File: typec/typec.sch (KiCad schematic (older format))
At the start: 26 parts, among them U1 TPD6E05U06-USON, U2 TPD4E05U06-USON, U3 TPS62081-WSON, U4 TPD4E05U06-USON, U5 TPS74801-VSON, U6 TUSB212-X2QFN

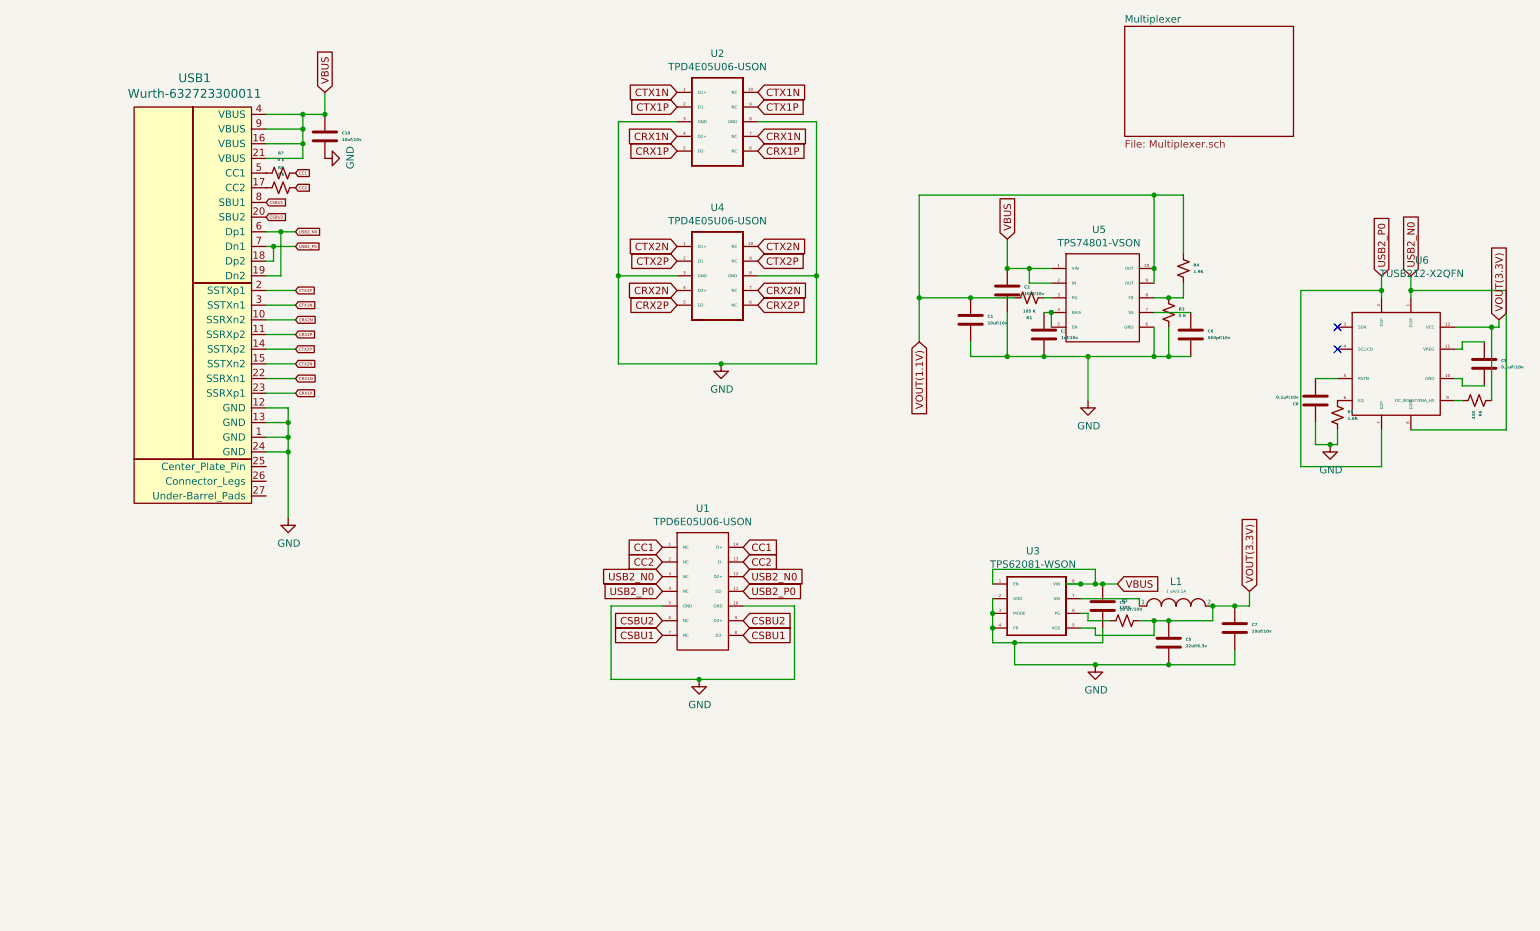
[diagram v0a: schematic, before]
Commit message: updated
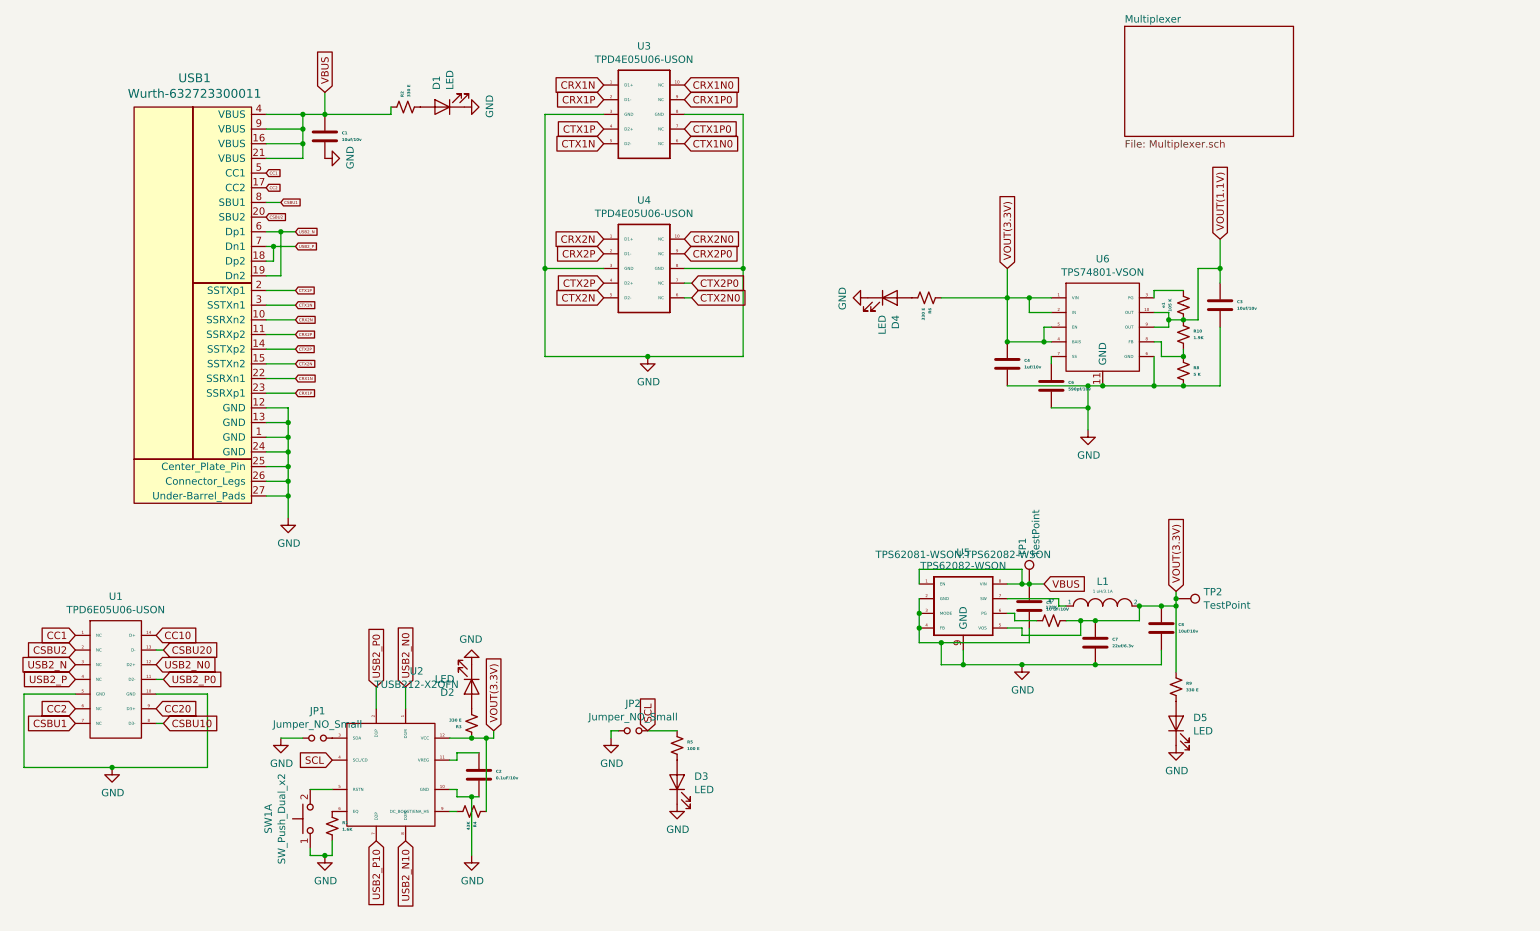
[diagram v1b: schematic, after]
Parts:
- removed C1: 10uf/10v, Capacitor_SMD:C_0805_2012Metric, symbol Device:C
- removed C9: 0.1uF/10v, Capacitor_SMD:C_0402_1005Metric, symbol Device:C
- removed U3: TPS62081-WSON, TPS62081-WSON:TPS62081-WSON, symbol typec-rescue:TPS62081-WSON-TPS62081-WSON
- removed U5: TPS74801-VSON, TPS74801-VSON:TPS74801-VSON, symbol typec-rescue:TPS74801-VSON-TPS74801-VSON
- removed U6: TUSB212-X2QFN, TUSB212-X2QFN:TUSB212-X2QFN, symbol TUSB212-X2QFN:TUSB212-X2QFN
- added D1, D2, D3, D4, D5: LED, LED_SMD:LED_0402_1005Metric, symbol Device:LED
- added JP1, JP2: Jumper_NO_Small, Connector_PinHeader_1.00mm:PinHeader_1x02_P1.00mm_Vertical, symbol Device:Jumper_NO_Small
- added R10: 1.9K, Resistor_SMD:R_0402_1005Metric, symbol Device:R_Small_US
- added R9: 330 E, Resistor_SMD:R_0402_1005Metric, symbol Device:R_Small_US
- added SW1: SW_Push_Dual_x2, Button_Switch_THT:SW_DIP_SPSTx01_Slide_6.7x4.1mm_W7.62mm_P2.54mm_LowProfile, symbol Switch:SW_Push_Dual_x2
- added TP1, TP2: TestPoint, TestPoint:TestPoint_THTPad_2.0x2.0mm_Drill1.0mm, symbol Connector:TestPoint
- added U2: TUSB212-X2QFN, TUSB212-X2QFN:TUSB212-X2QFN, symbol TUSB212-X2QFN:TUSB212-X2QFN
- added U5: TPS62082-WSON, TPS62081-WSON:TPS62082-WSON, symbol typec-rescue:TPS62082-WSON
- added U6: TPS74801-VSON, TPS74801-VSON:TPS74801-VSON, symbol TPS74801-VSON:TPS74801-VSON
- added e1: 105 K, Resistor_SMD:R_0201_0603Metric, symbol Device:R_Small_US
- C2: value 10uf/10v -> 0.1uF/10v; footprint Capacitor_SMD:C_0805_2012Metric -> Capacitor_SMD:C_0402_1005Metric
- C3: value 1uf/10v -> 10uf/10v
- C4: value 10 uF/10V -> 1uf/10v; footprint Capacitor_SMD:C_0805_2012Metric -> Capacitor_SMD:C_0603_1608Metric
- C5: value 22uf/6.3v -> 10 uF/10V; footprint Capacitor_SMD:C_0805_2012Metric -> Capacitor_SMD:C_0603_1608Metric
- C6: value 560pf/10v -> 590pf/10v; footprint Capacitor_SMD:C_0402_1005Metric -> Capacitor_SMD:C_0201_0603Metric
- C7: value 10uf/10v -> 22uf/6.3v; footprint Capacitor_SMD:C_0805_2012Metric -> Capacitor_SMD:C_0603_1608Metric
- C8: value 0.1uF/10v -> 10uf/10v; footprint Capacitor_SMD:C_0402_1005Metric -> Capacitor_SMD:C_0603_1608Metric
- R1: value 105 K -> 1.6K; footprint Resistor_SMD:R_0805_2012Metric -> Resistor_SMD:R_0201_0603Metric
- R2: value 178K -> 330 E; footprint Resistor_SMD:R_0805_2012Metric -> Resistor_SMD:R_0402_1005Metric
- R3: value 5 K -> 330 E; footprint Resistor_SMD:R_0805_2012Metric -> Resistor_SMD:R_0201_0603Metric
- R4: value 1.9K -> 43K; footprint Resistor_SMD:R_0805_2012Metric -> Resistor_SMD:R_0201_0603Metric
- R5: value 1.6K -> 100 E; footprint Resistor_SMD:R_0805_2012Metric -> Resistor_SMD:R_0402_1005Metric
- R6: value 43K -> 330 E; footprint Resistor_SMD:R_0805_2012Metric -> Resistor_SMD:R_0402_1005Metric
- R7: value 0 E -> 178K; footprint Resistor_SMD:R_0805_2012Metric -> Resistor_SMD:R_0402_1005Metric
- R8: value 0 E -> 5 K; footprint Resistor_SMD:R_0805_2012Metric -> Resistor_SMD:R_0402_1005Metric
- renumbered C10 to C1, U2 to U3
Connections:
- net CC1: now also USB1.5 (CC1); no longer R7.1, U1.14 (D+)
- net CC2: now also U1.6 (NC), USB1.17 (CC2); no longer R8.1, U1.13 (D-), U1.2 (NC)
- net CRX1N: now also U3.1 (D1+); no longer U3.4 (D2+), U3.7 (NC)
- net CRX1P: now also U3.2 (D1-); no longer U3.5 (D2-), U3.6 (NC)
- net CRX2N: now also U4.1 (D1+); no longer U4.4 (D2+), U4.7 (NC)
- net CRX2P: now also U4.2 (D1-); no longer U4.5 (D2-), U4.6 (NC)
- net CSBU1: no longer U1.8 (D3-)
- net CSBU2: now also U1.2 (NC); no longer U1.6 (NC), U1.9 (D3+)
- net CTX1N: now also U3.5 (D2-); no longer U3.1 (D1+), U3.10 (NC)
- net CTX1P: now also U3.4 (D2+); no longer U3.2 (D1-), U3.9 (NC)
- net CTX2N: now also U4.5 (D2-); no longer U4.1 (D1+), U4.10 (NC)
- net CTX2P: now also U4.4 (D2+); no longer U4.2 (D1-), U4.9 (NC)
- net GND: now also C8.2, R1.2, R8.1, USB1.25 (Center_Plate_Pin), USB1.26 (Connector_Legs), USB1.27 (Under-Barrel_Pads), D1.1 (K), D2.1 (K), D3.1 (K), D4.1 (K), D5.1 (K), JP1.1, JP2.1, SW1.1 (C), U2.10 (GND), U5.2 (GND), U5.3 (MODE), U5.4 (FB), U5.9 (GND), U6.11 (GND), U6.6 (GND); no longer C8.1, R3.1, R5.2
- net USB2_N0: now also U2.1 (D1M); no longer U1.3 (NC), USB1.19 (Dn2), USB1.6 (Dp1)
- net USB2_P0: now also U2.2 (D1P); no longer U1.4 (NC), USB1.18 (Dp2), USB1.7 (Dn1)
- net VBUS: now also C5.1, R2.1, TP1.1, U5.1 (EN), U5.8 (VIN); no longer C2.1, C4.1
- net VOUT(1.1V): now also C3.1, R10.1, U6.10 (OUT), U6.9 (OUT), e1.2; no longer R1.1, R4.1
- net VOUT(3.3V): now also C4.1, C8.1, R3.1, R4.1, R7.2, R9.1, TP2.1, U2.12 (VCC), U5.5 (VOS), U6.1 (VIN), U6.2 (IN), U6.4 (BAIS), U6.5 (EN); no longer C5.1, R2.2
- net at L1.1: now also U5.7 (SW)
- net at C6.1: now also U6.7 (SS)
- net at R3.2: now also D2.2 (A); no longer R4.2
- net SCL: now reaches R5.1
- net SCL: now also JP2.2, U2.4 (SCL/CD)
- net at R6.2: now also D4.2 (A)
- net at R8.2: now also R10.2, U6.8 (FB); no longer USB1.17 (CC2)
- new net: U6.3 (PG), e1.1
- new net: SW1.2 (D), U2.5 (RSTN)
- new net: JP1.2, U2.3 (SDA)
- new net: R1.1, U2.6 (EQ)
- new net: R4.2, U2.9 (DC_BOOST/ENA_HS)
- new net: C2.1, U2.11 (VREG)
- new net: D3.2 (A), R5.2
- new net: R7.1, U5.6 (PG)
- new net: D5.2 (A), R9.2
- new net: D1.2 (A), R2.2
- new net CC10: U1.14 (D+)
- new net CC20: U1.9 (D3+)
- new net CRX1N0: U3.10 (NC)
- new net CRX1P0: U3.9 (NC)
- new net CRX2N0: U4.10 (NC)
- new net CRX2P0: U4.9 (NC)
- new net CSBU10: U1.8 (D3-)
- new net CSBU20: U1.13 (D-)
- new net CTX1N0: U3.6 (NC)
- new net CTX1P0: U3.7 (NC)
- new net CTX2N0: U4.6 (NC)
- new net CTX2P0: U4.7 (NC)
- new net USB2_N: U1.3 (NC), USB1.19 (Dn2), USB1.6 (Dp1)
- new net USB2_N10: U2.8 (D2M)
- new net USB2_P: U1.4 (NC), USB1.18 (Dp2), USB1.7 (Dn1)
- new net USB2_P10: U2.7 (D2P)
- no-connect marks 2 -> 0
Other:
- moved on the sheet: U1, U3, U4

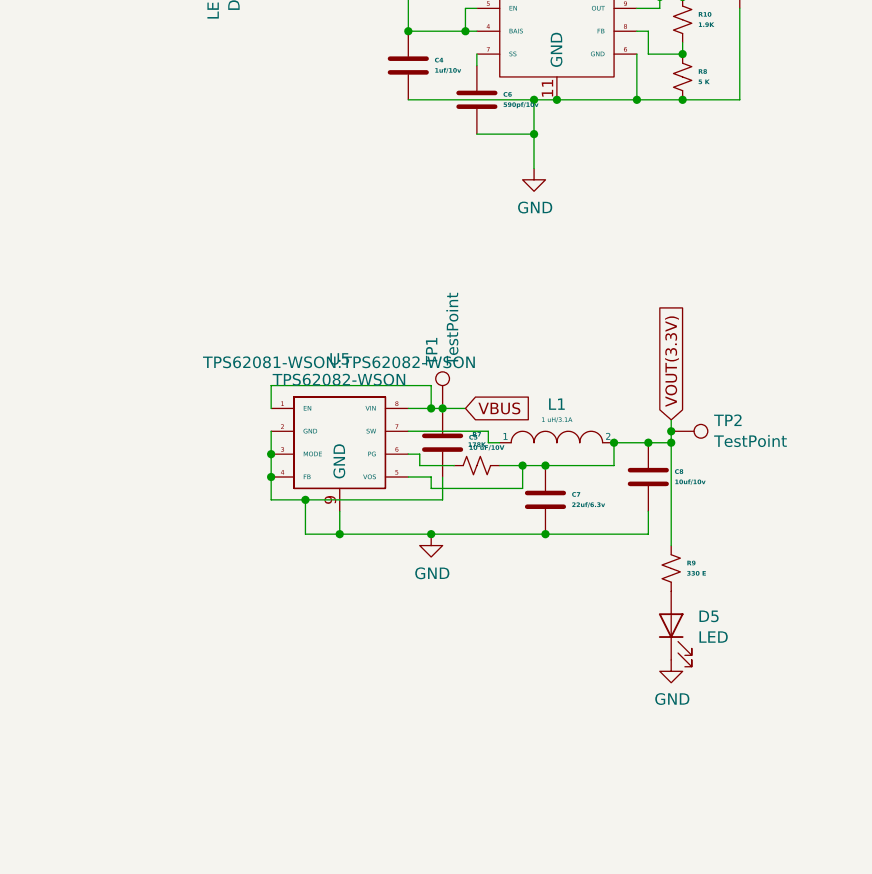
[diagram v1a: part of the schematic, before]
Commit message: 2.0
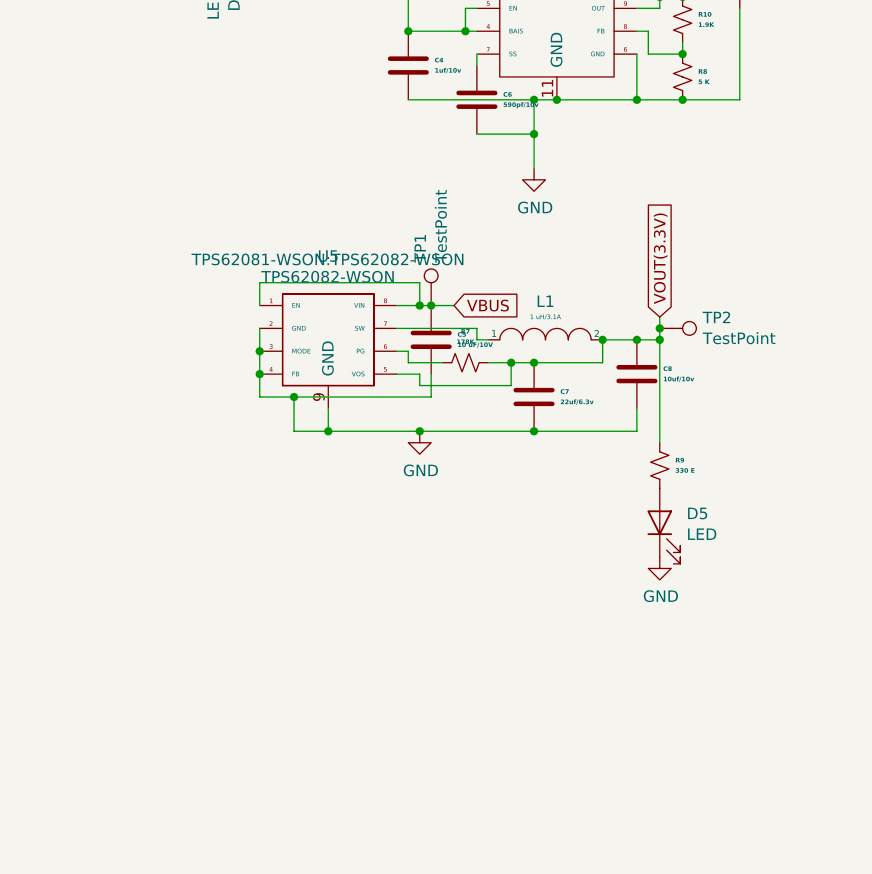
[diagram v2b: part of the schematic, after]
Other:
- moved on the sheet: C5, C7, C8, D5, L1, R7, R9, TP1, TP2, U5
